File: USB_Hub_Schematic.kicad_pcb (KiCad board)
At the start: 4 copper layers, 43.5 x 88 mm, 108 parts, among them J1 USB-C, J2 USB-A, U1 USB2517 Chip, U10 TP, U11 TP, U12 TP, U13 TP, U14 TP, U15 TP, U16 TPS25821, U17 TPS25821, U2 3.3V CONV, U3 MUX, U4 USB to microSD, U7 TPS2052B, U9 TP, X3 24MHz Osc

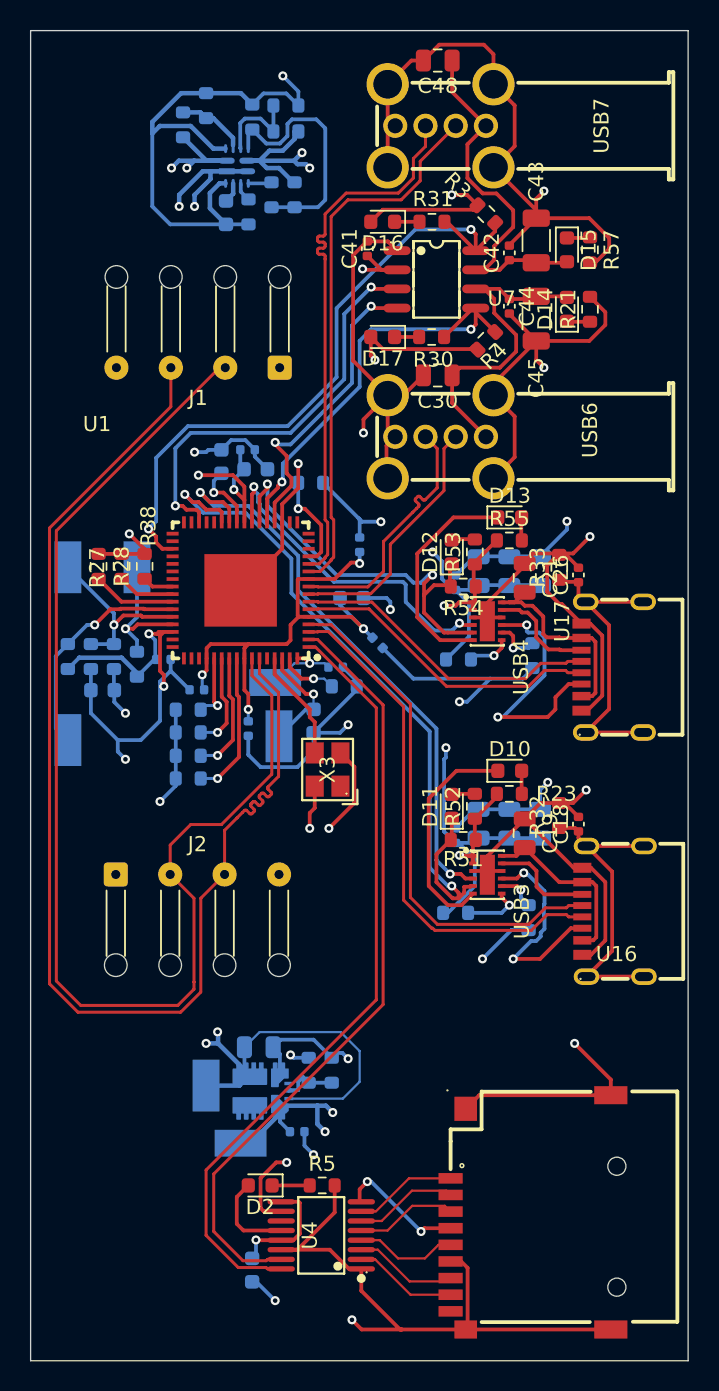
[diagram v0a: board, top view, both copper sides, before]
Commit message: Routing Updates
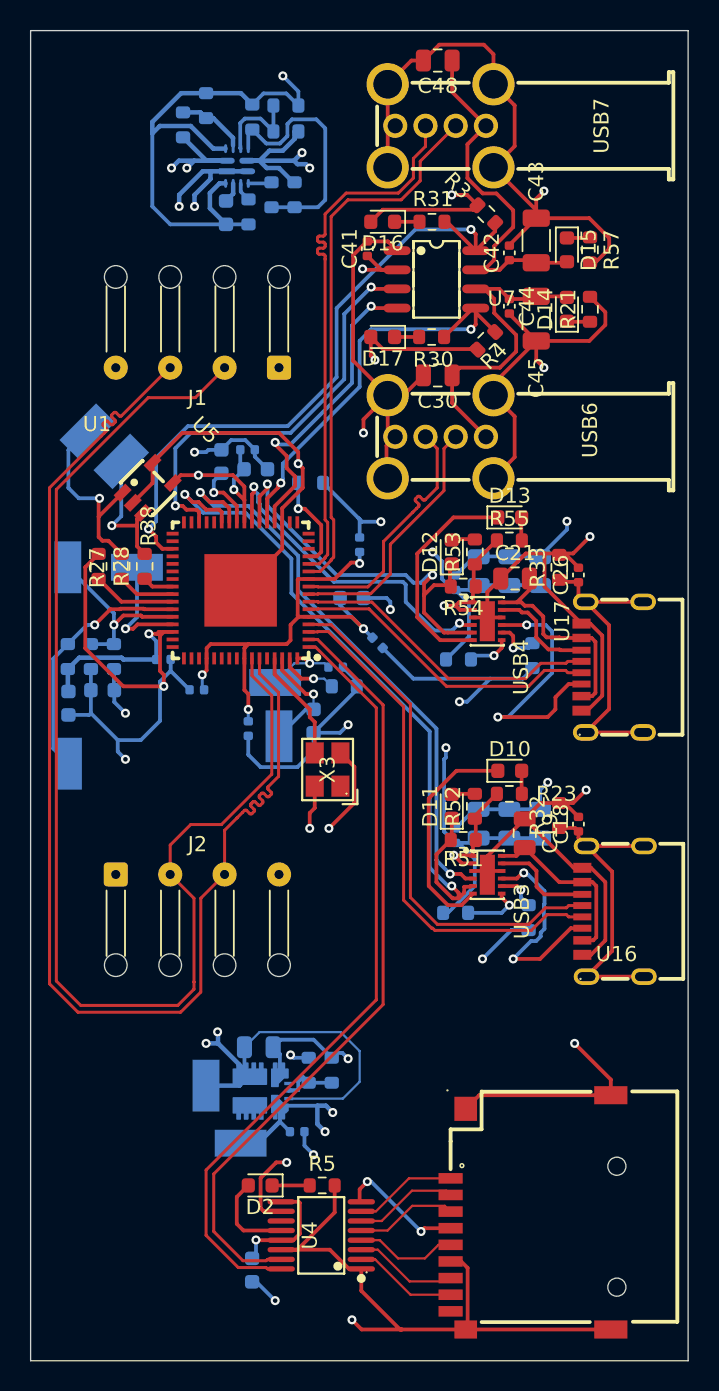
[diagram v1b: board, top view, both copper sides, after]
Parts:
- removed R24, R25, R26, R42, R46: 10k, Resistor_SMD:R_0603_1608Metric
- added C5: 1 uF, Capacitor_SMD:C_0603_1608Metric, B.Cu at (124.8, 73.0)
- added U18: TP, lcsc_easyeda:TEST-SMD_L2.7-W1.0, B.Cu at (126.0, 55.0)
- added U19: TP, lcsc_easyeda:TEST-SMD_L2.7-W1.0, B.Cu at (128.2, 57.0)
- added U5: 24AA02, lcsc_easyeda:SOT-23-5_L2.9-W1.6-P0.95-LS2.8-BL-3, F.Cu at (130.0, 58.8)
- moved U15 1.56 mm to (124.8, 77.0)
- moved C21 0.64 mm to (154.3, 64.8), turned to 0 degrees
- turned U13 to 180 degrees
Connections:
- R27 pad 2: GND -> /3.3V_GLOBAL
- R28 pad 2: GND -> /EEPROM_CLK
- R38 pad 2: GND -> /EEPROM_DATA
- U1 pad 53: Net-(U1-USBDN6_DM/PRT_DIS_M6) -> unconnected-(U1-USBDN6_DM/PRT_DIS_M6-Pad53)
- U1 pad 54: Net-(U1-USBDN6_DP/PRT_DIS_P6) -> unconnected-(U1-USBDN6_DP/PRT_DIS_P6-Pad54)
- U1 pad 55: Net-(U1-USBDN7_DM/PRT_DIS_M7) -> unconnected-(U1-USBDN7_DM/PRT_DIS_M7-Pad55)
- U1 pad 56: Net-(U1-USBDN7_DP/PRT_DIS_P7) -> unconnected-(U1-USBDN7_DP/PRT_DIS_P7-Pad56)
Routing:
- net /EEPROM_CLK: track 0.00 -> 13.4 mm, vias 0 -> 1
- net GND: track 346.8 -> 358.0 mm, vias 22 -> 21
- net Net-(U1-USBDN7_DP/PRT_DIS_P7): track 9.71 -> 0.00 mm, vias 1 -> 0
- net /EEPROM_DATA: track 0.00 -> 9.26 mm, vias 0 -> 1
- net /3.3V_GLOBAL: track 296.6 -> 305.3 mm, vias 11 -> 10
- net Net-(U1-USBDN7_DM/PRT_DIS_M7): track 8.07 -> 0.00 mm, vias 1 -> 0
- net Net-(U1-USBDN6_DP/PRT_DIS_P6): track 6.40 -> 0.00 mm, vias 1 -> 0
- net Net-(U1-USBDN6_DM/PRT_DIS_M6): track 4.45 -> 0.00 mm, vias 1 -> 0
- net /TP_SUSPIND: track 9.46 -> 7.62 mm
- net /TP_RESET: track 14.9 -> 16.6 mm
- net /UP_DP: track 82.6 -> 84.3 mm
- net /UP_DN: track 82.7 -> 84.3 mm
- net /C2_CC1: track 17.0 -> 18.0 mm
- net /PORT3: track 13.7 -> 14.3 mm
